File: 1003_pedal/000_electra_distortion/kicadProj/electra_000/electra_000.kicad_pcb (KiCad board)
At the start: 2 copper layers, 17 parts, among them J1 AudioJack2, J2 AudioJack2, Q1 Q_NPN_BCE, SW1 SW_Slide_DPDT

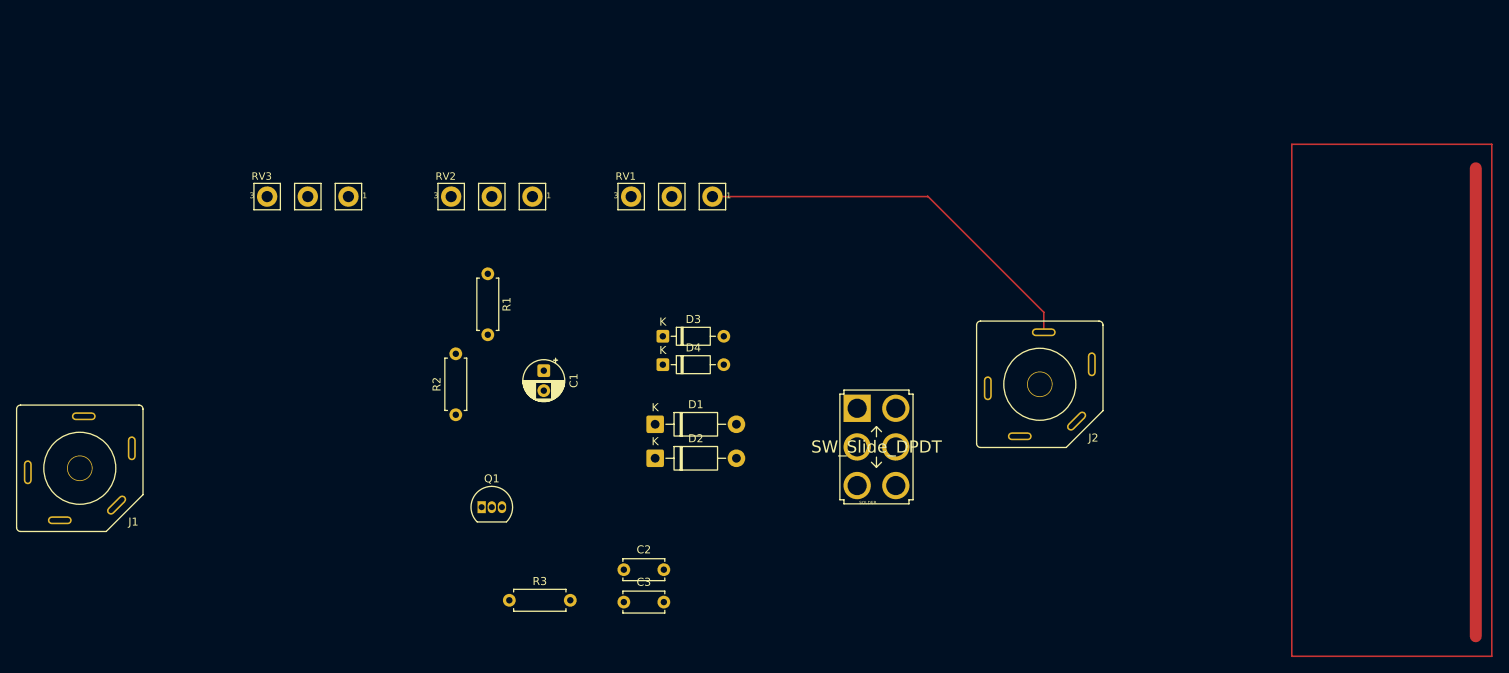
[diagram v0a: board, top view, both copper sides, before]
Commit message: schematic
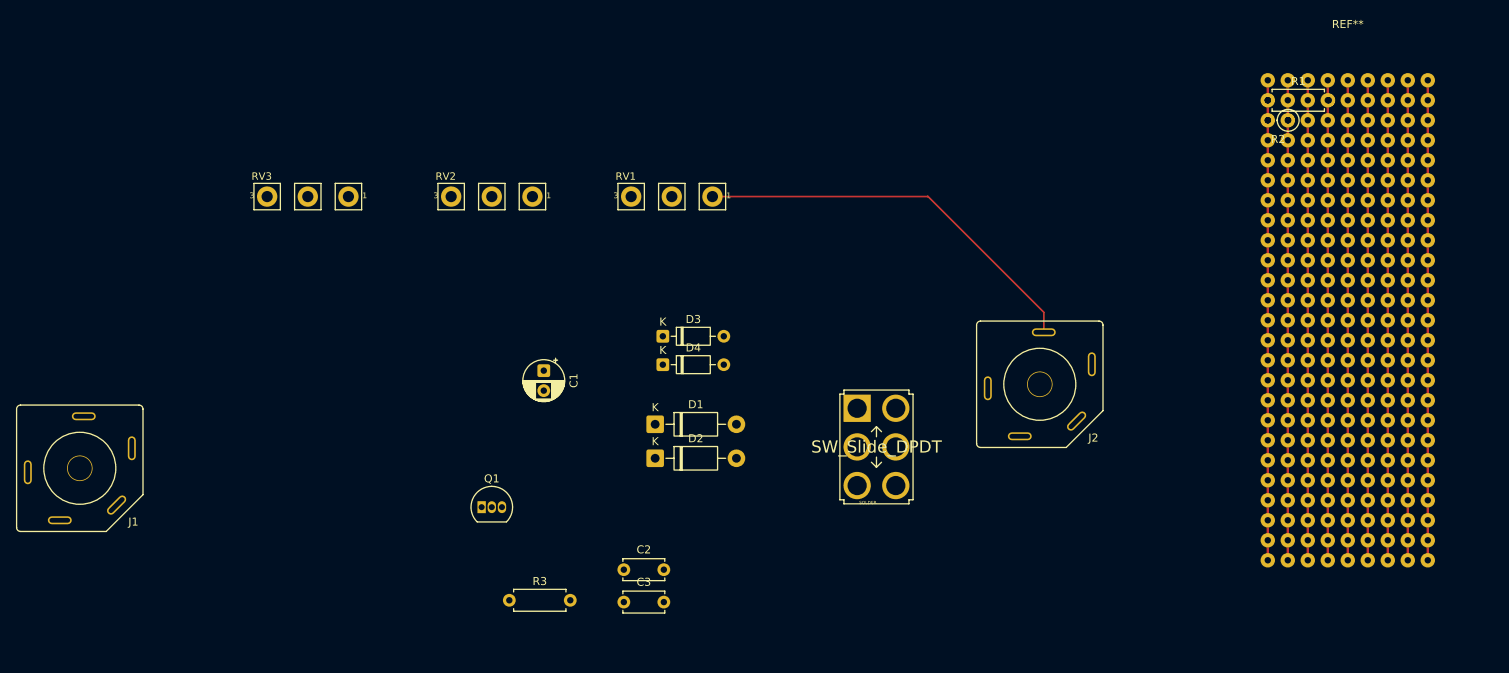
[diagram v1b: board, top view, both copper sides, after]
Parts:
- added REF**: VeroBoard_25x64, VeroBoard:Veroboard_25x64, F.Cu at (202.5, 72.0)
- R2: footprint Resistor_THT:R_Axial_DIN0207_L6.3mm_D2.5mm_P7.62mm_Horizontal -> Resistor_THT:R_Axial_DIN0207_L6.3mm_D2.5mm_P2.54mm_Vertical
- moved R2 110.4 mm to (195.0, 47.0), turned to 180 degrees
- moved R1 99.9 mm to (192.5, 44.5), turned to 0 degrees
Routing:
- net (no net): track 58.5 -> 0.00 mm
